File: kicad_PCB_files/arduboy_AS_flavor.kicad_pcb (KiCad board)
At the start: 2 copper layers, 50.6 x 82.6 mm, 86 parts, among them J1 SSD1306_SSH1106, J2 Expansion_port_NEW, J3 USB_B_Micro, Q1 2N7002, Q2 Si2301CDS, SW1 RST Button, SW2 UP Button, SW3 DOWN Button, SW4 LEFT Button, SW5 RIGHT Button, SW6 A Button, SW7 B Button, U1 ATmega32U4-AU, U2 W25Q128JVSIQ, U3 XC6206P33, U4 TP4054, U5 MPU-6050, Y1 16MHz

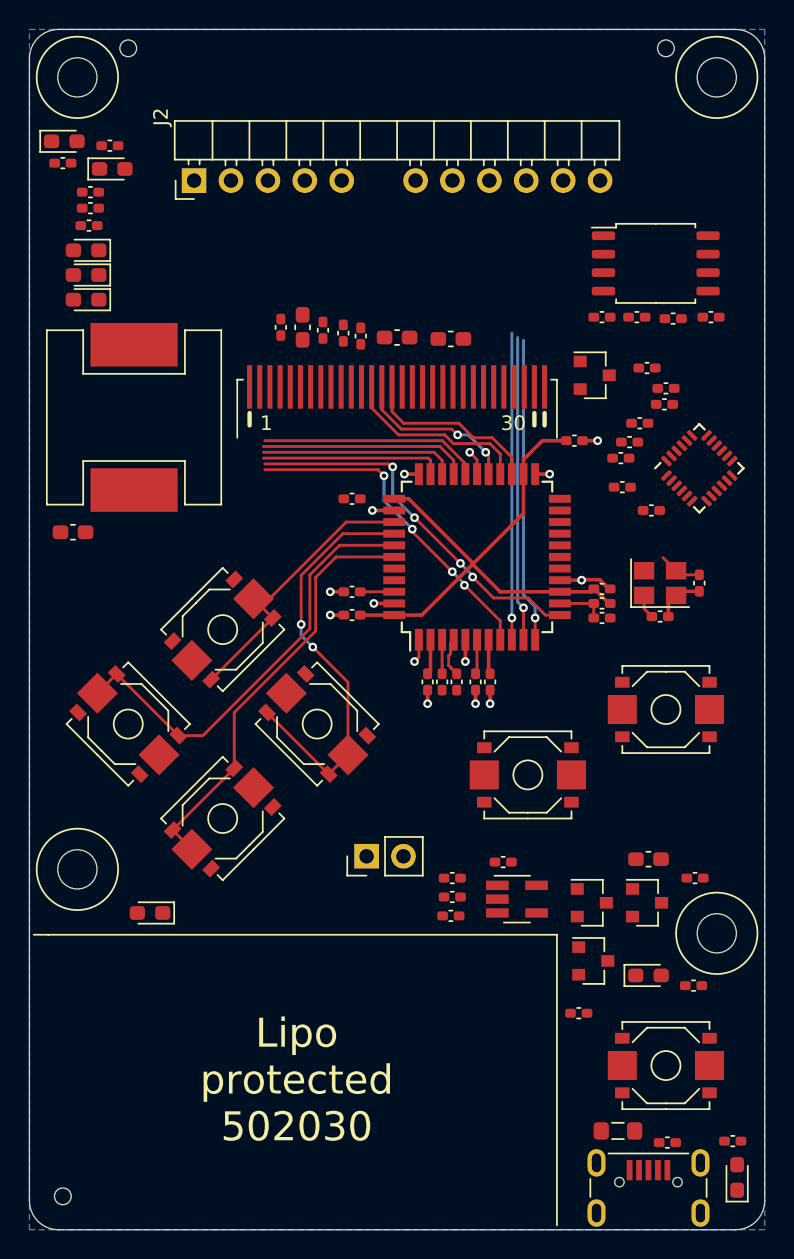
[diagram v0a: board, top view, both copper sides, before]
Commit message: Major changes, practically v2
Changed board shape
Changed a great part of the schematic
Component placement done
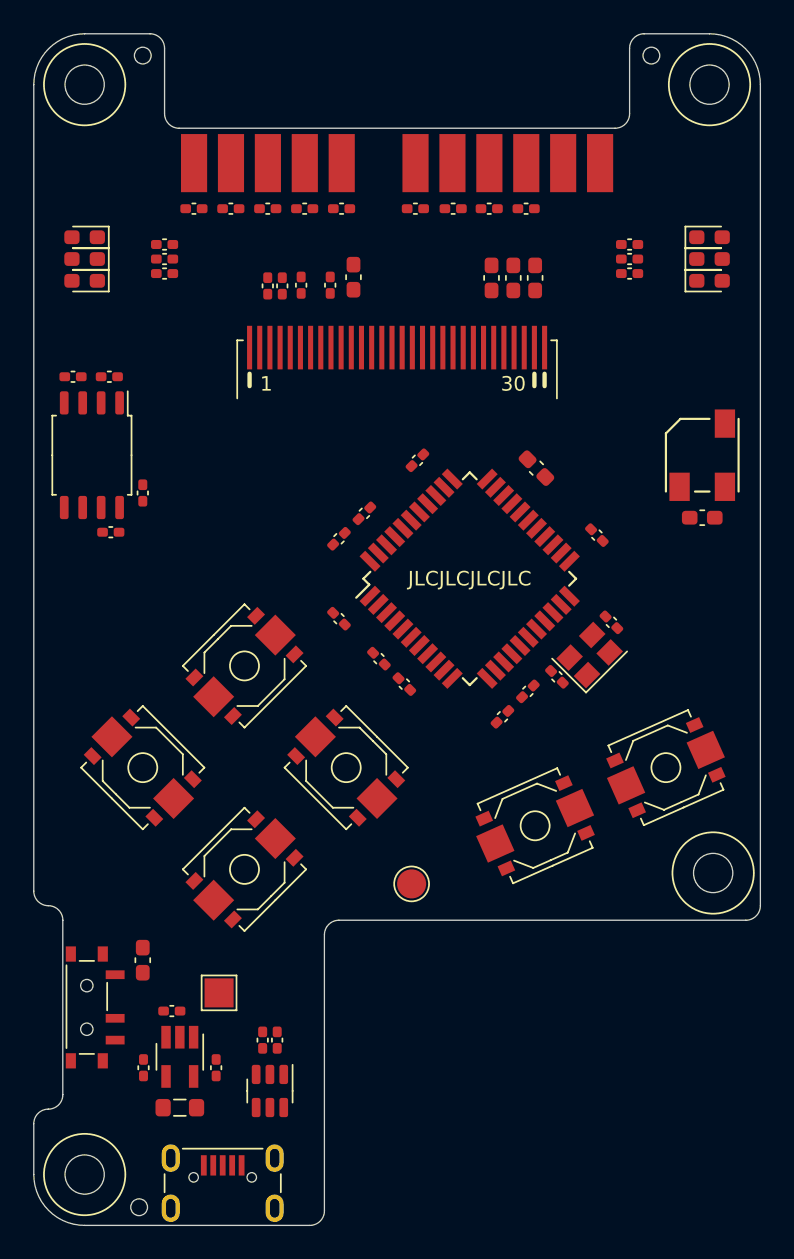
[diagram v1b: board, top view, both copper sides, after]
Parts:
- removed C23: 10nF, no_refdes:0402_HandSolder
- removed C24, C26: 100nF, no_refdes:0402_HandSolder
- removed C25: 2.2nF, no_refdes:0402_HandSolder
- removed C27: 1uF, no_refdes:0402_HandSolder
- removed D1: BAV70, Package_TO_SOT_SMD:SOT-23
- removed D5, D6: Yellow, LED_SMD:LED_0603_1608Metric_Pad1.05x0.95mm_HandSolder
- removed JP1: Speaker, arduboy:CPT-12123-81-SMT
- removed JP2: LiPo, Connector_PinHeader_2.54mm:PinHeader_1x02_P2.54mm_Vertical
- removed Q1: 2N7002, Package_TO_SOT_SMD:SOT-23
- removed Q2: Si2301CDS, Package_TO_SOT_SMD:SOT-23
- removed R15: 220, no_refdes:0603_HandSolder
- removed U5: MPU-6050, Sensor_Motion:InvenSense_QFN-24_4x4mm_P0.5mm
- added BZ1: Buzzer, arduboy:Buzzer_KLJ-5020, F.Cu at (68.0, 51.0)
- added R22: 120, no_refdes:0402_HandSolder, F.Cu at (50.9, 34.0)
- added R23: 120, no_refdes:0402_HandSolder, F.Cu at (53.3, 34.0)
- added R24: 120, no_refdes:0402_HandSolder, F.Cu at (55.9, 34.0)
- added TP1: Lipo [+], TestPoint:TestPoint_Pad_2.0x2.0mm, F.Cu at (34.8, 88.0)
- added TP16: Lipo (-), TestPoint:TestPoint_Pad_D2.0mm, F.Cu at (48.0, 80.5)
- C1: value 100nF -> 10uF; footprint no_refdes:0402_HandSolder -> no_refdes:0603_HandSolder
- C15: value 2.2uF -> 4.7uF
- C8: value 1uF -> 10uF; footprint no_refdes:0402_HandSolder -> no_refdes:0603_HandSolder
- C9: value 1uF -> 4.7uF; footprint no_refdes:0402_HandSolder -> no_refdes:0603_HandSolder
- J1: value SSD1306_SSH1106 -> SSD1306
- J2: footprint arduboy:PinHeader_1x12_P2.54mm_SLOTTED_ROTATED -> arduboy:ExpansionPort_SMD
- R12: value 6.8k -> 1.2k
- R13: value 3.3k -> 1.2k
- R14: value 3.3k -> 4.7k
- R18, R19: value 4.7k -> 120
- R5, R8: value 10k -> 120
- R6: value 6.8k -> 120
- R7: value 3.3k -> 120
- SW1: value RST Button -> ON/OFF; footprint arduboy:button_TS-1187A-B-A-B -> arduboy:Switch_DPDT_MSK12CO2-BDM
- U3: value XC6206P33 -> SRV05-4; footprint Package_TO_SOT_SMD:SOT-23 -> Package_TO_SOT_SMD:SOT-23-6
- moved H5 87.1 mm to (25.5, 100.5)
- moved R6 72.9 mm to (35.6, 34.0), turned to 180 degrees
- moved R5 61.4 mm to (33.0, 34.0), turned to 180 degrees
- moved R7 61.0 mm to (38.1, 34.0), turned to 180 degrees
- moved D7 60.4 mm to (68.5, 36.0), turned to 0 degrees
- moved U3 54.1 mm to (38.2, 94.8), turned to -90 degrees
- moved H7 54.0 mm to (25.5, 25.5)
- moved R8 53.3 mm to (40.6, 34.0), turned to 180 degrees
- moved D8 45.1 mm to (68.5, 37.5)
- moved C7 44.9 mm to (44.0, 38.8), turned to 90 degrees
- moved R12 44.3 mm to (63.0, 37.5), turned to 180 degrees
- moved H4 43.5 mm to (68.5, 25.5)
- moved D9 41.8 mm to (68.5, 39.0)
- moved R3 41.5 mm to (24.7, 45.6), turned to 180 degrees
- moved U2 41.0 mm to (26.0, 51.0), turned to -90 degrees
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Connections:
- net /~HOLD renamed /~{HOLD}
- net /~WP renamed /~{WP}
- net Net-(R16-Pad1) renamed /PROG
- C1 pad 1: RST -> VCC
- C1 pad 2: Net-(C1-Pad2) -> GND
- C9 pad 1: +3V3 -> SPKR1
- C9 pad 2: GND -> Net-(BZ1-Pad1)
- D7 pad 2: Net-(D7-Pad2) -> +5V
- D8 pad 1: GND -> Net-(D8-Pad1)
- D8 pad 2: Net-(D8-Pad2) -> VCC
- D9 pad 1: GND -> Net-(D9-Pad1)
- D9 pad 2: Net-(D9-Pad2) -> VCC
- J1 pad 1: Net-(J1-Pad1) -> unconnected-(J1-Pad1)
- J1 pad 20: Net-(J1-Pad20) -> unconnected-(J1-Pad20)
- J1 pad 21: Net-(J1-Pad21) -> unconnected-(J1-Pad21)
- J1 pad 22: Net-(J1-Pad22) -> unconnected-(J1-Pad22)
- J1 pad 23: Net-(J1-Pad23) -> unconnected-(J1-Pad23)
- J1 pad 24: Net-(J1-Pad24) -> unconnected-(J1-Pad24)
- J1 pad 25: Net-(J1-Pad25) -> unconnected-(J1-Pad25)
- J1 pad 29: Net-(J1-Pad29) -> unconnected-(J1-Pad29)
- J1 pad 30: Net-(J1-Pad30) -> unconnected-(J1-Pad30)
- J2 pad 10: SCL_3V3 -> Net-(J2-Pad10)
- J2 pad 11: SDA+FCS -> Net-(J2-Pad11)
- J2 pad 12: TX -> Net-(J2-Pad12)
- J2 pad 3: RST -> Net-(J2-Pad3)
- J2 pad 4: SCLK -> Net-(J2-Pad4)
- J2 pad 5: MOSI -> Net-(J2-Pad5)
- J2 pad 6: MISO -> Net-(J2-Pad6)
- J2 pad 8: A5 -> Net-(J2-Pad8)
- J2 pad 9: RX -> Net-(J2-Pad9)
- J3 pad 4: Net-(J3-Pad4) -> unconnected-(J3-Pad4)
- J3 pad 6: Net-(J3-Pad6) -> unconnected-(J3-Pad6)
- R12 pad 1: +5V -> Net-(D8-Pad1)
- R12 pad 2: Net-(D7-Pad2) -> RX_LED
- R13 pad 1: RX_LED -> Net-(D9-Pad1)
- R13 pad 2: Net-(D8-Pad2) -> TX_LED
- R14 pad 1: TX_LED -> Net-(D7-Pad1)
- R14 pad 2: Net-(D9-Pad2) -> ~{CHRG}
- R18 pad 1: +3V3 -> A5
- R18 pad 2: SCL_3V3 -> Net-(J2-Pad8)
- R19 pad 1: +3V3 -> MISO
- R19 pad 2: SDA+FCS -> Net-(J2-Pad6)
- R5 pad 1: EN -> TX
- R5 pad 2: GND -> Net-(J2-Pad12)
- R6 pad 1: +5V -> SDA+FCS
- R6 pad 2: Net-(D5-Pad2) -> Net-(J2-Pad11)
- R7 pad 1: VCC -> SCL
- R7 pad 2: Net-(D6-Pad2) -> Net-(J2-Pad10)
- R8 pad 1: +BATT -> RX
- R8 pad 2: ~PWR_EN -> Net-(J2-Pad9)
- SW1 pad 1: GND -> VCC
- SW1 pad 2: Net-(D1-Pad3) -> +BATT
- U1 pad 18: SCL_3V3 -> SCL
- U1 pad 40: EN -> A4
- U3 pad 1: GND -> /USB_D+
- U3 pad 2: +3V3 -> GND
- U3 pad 3: VCC -> /USB_D-
- U4 pad 1: Net-(D7-Pad1) -> ~{CHRG}
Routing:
- net VCC: track 39.4 -> 0.00 mm
- net Btn_LEFT: track 30.3 -> 0.00 mm
- net Btn_DOWN: track 29.3 -> 0.00 mm
- net Btn_RIGHT: track 29.2 -> 0.00 mm, vias 2 -> 0
- net LED_G: track 25.8 -> 0.00 mm, vias 4 -> 0
- net RX_LED: track 23.0 -> 0.00 mm, vias 4 -> 0
- net SCK: track 21.1 -> 0.00 mm, vias 1 -> 0
- net MOSI: track 21.0 -> 0.00 mm, vias 1 -> 0
- net MISO: track 20.9 -> 0.00 mm, vias 1 -> 0
- net Btn_UP: track 19.7 -> 0.00 mm
- net GND: track 19.2 -> 0.00 mm, vias 12 -> 0
- net LED_B: track 15.2 -> 0.00 mm
- net LED_R: track 14.4 -> 0.00 mm
- net SPKR1: track 13.5 -> 0.00 mm
- net OLED_CS: track 13.0 -> 0.00 mm
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- added copper zone on In1.Cu, net GND
- removed copper zone on B.Cu, net GND
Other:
- board size 50.6 x 82.6 mm -> 50 x 82 mm
- copper layers 2 -> 4
- net class Default removed
- net class Power removed
- board text added: "JLCJLCJLCJLC"
